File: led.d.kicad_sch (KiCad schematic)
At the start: 4 parts, among them J1 USB_B_Micro, J2 Conn_02x02_Top_Bottom

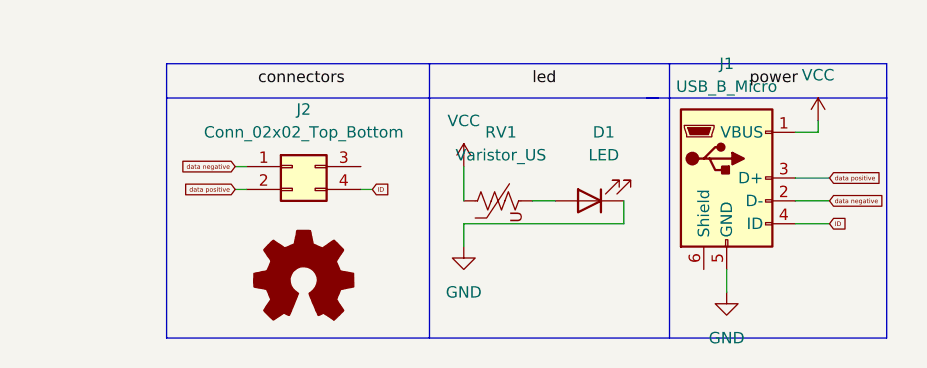
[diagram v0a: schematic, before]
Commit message: update
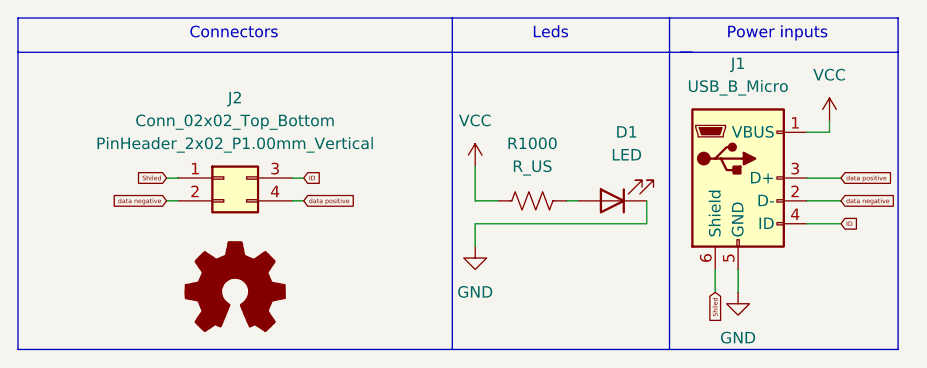
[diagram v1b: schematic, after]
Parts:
- removed RV1: Varistor_US, Varistor:RV_Disc_D7mm_W3.4mm_P5mm, symbol Device:Varistor_US
- added R1000: R_US, Resistor_THT:R_Axial_DIN0204_L3.6mm_D1.6mm_P5.08mm_Horizontal, symbol Device:R_US
- J2: footprint Conn_02x02_Top_Bottom:Conn_02x02_Top_Bottom -> PinHeader_2x02_P1.00mm_Vertical
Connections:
- net ID: now also J2.3 (Pin_3); no longer J2.4 (Pin_4)
- net VCC: now also R1000.1
- net data negative: now also J2.2 (Pin_2); no longer J2.1 (Pin_1)
- net data positive: now also J2.4 (Pin_4); no longer J2.2 (Pin_2)
- net at D1.2 (A): now also R1000.2
- net Shiled: now reaches J1.6 (Shield)
- net Shiled: now also J2.1 (Pin_1)
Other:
- note added: "Connectors"
- note added: "Leds"
- note added: "Power inputs"
- moved on the sheet: D1, J1, J2
